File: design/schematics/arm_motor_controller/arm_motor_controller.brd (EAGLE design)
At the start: 97.2 x 54.6 mm, 65 parts, among them Q1 PFET-FQP27P06, Q2 PFET-FQP27P06, Q3 NFET-FQP30N06L, Q4 NFET-FQP30N06L, Q5 PFET-FQP27P06, Q6 PFET-FQP27P06, Q7 NFET-FQP30N06L, Q8 NFET-FQP30N06L

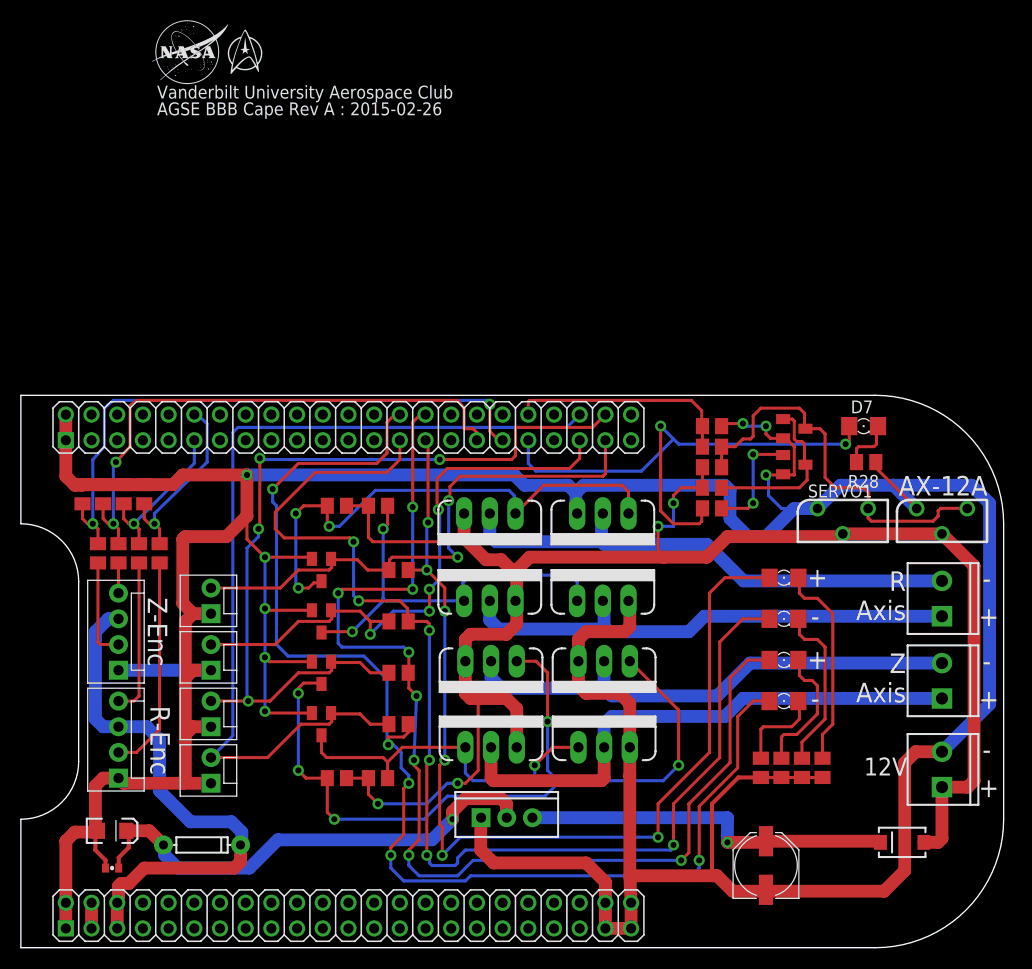
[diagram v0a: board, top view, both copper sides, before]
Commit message: working on updating the board routing.
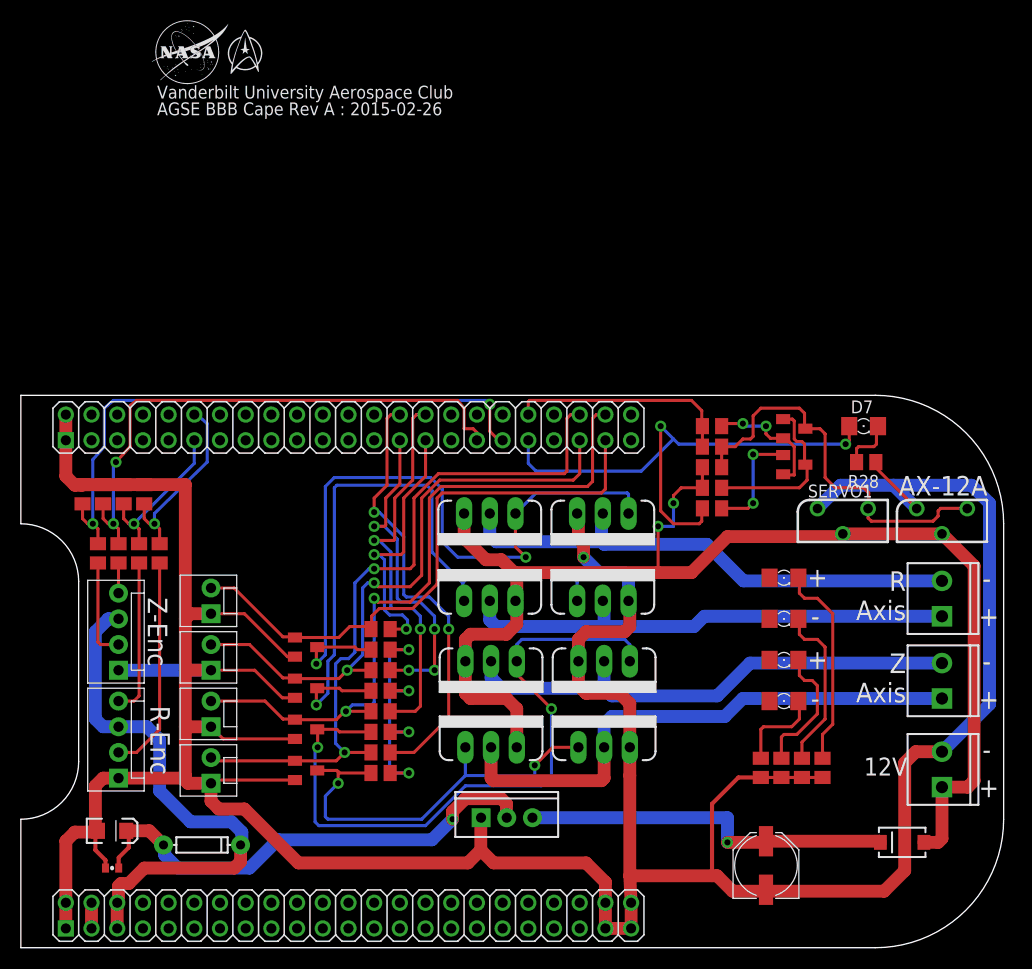
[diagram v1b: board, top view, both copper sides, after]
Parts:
- moved R8 18.3 mm to (39.6, 25.7), turned to 0 degrees
- moved R9 14.9 mm to (39.6, 29.7)
- moved T4 7.77 mm to (32.3, 30.0), turned to 270 degrees
- moved T3 6.78 mm to (32.3, 25.9), turned to 270 degrees
- moved R5 6.29 mm to (39.6, 21.6)
- moved R11 6.11 mm to (39.6, 31.8)
- moved T2 5.79 mm to (32.3, 21.8), turned to 270 degrees
- moved R10 5.14 mm to (39.6, 27.7)
- moved T1 4.82 mm to (32.3, 17.8), turned to 270 degrees
- moved R7 4.20 mm to (39.6, 23.6)
- moved R6 3.31 mm to (39.6, 19.6)
- moved R4 0.57 mm to (39.6, 17.5), turned to 0 degrees
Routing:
- net -RADIUS: track 118.1 -> 32.9 mm, vias 6 -> 4
- net -HEIGHT: track 121.5 -> 43.4 mm, vias 5 -> 2
- net +HEIGHT: track 112.7 -> 39.1 mm, vias 8 -> 2
- net +RADIUS: track 99.0 -> 26.4 mm, vias 6 -> 2
- net GND: track 416.1 -> 372.8 mm, vias 8 -> 3
- net N$13: track 40.7 -> 65.3 mm, vias 2 -> 1
- net N$14: track 52.3 -> 70.4 mm, vias 3 -> 2
- net -HEIGHT_LS: track 88.5 -> 70.7 mm, vias 0 -> 2
- net N$8: track 81.6 -> 67.9 mm, vias 5 -> 2
- net +HEIGHT_LS: track 82.5 -> 69.6 mm, vias 4 -> 2
- net 12V: track 166.5 -> 156.2 mm, vias 4 -> 6
- net N$7: track 34.5 -> 41.9 mm, vias 1 -> 2
- net +RADIUS_LS: track 54.3 -> 57.8 mm, vias 2 -> 0
- net -RADIUS_LS: track 58.4 -> 60.5 mm, vias 4 -> 2
- net R+: track 50.5 -> 49.9 mm
